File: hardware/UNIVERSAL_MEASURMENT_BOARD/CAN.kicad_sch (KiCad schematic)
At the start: 12 parts, among them U5 ADM3055EBRIZ-RL

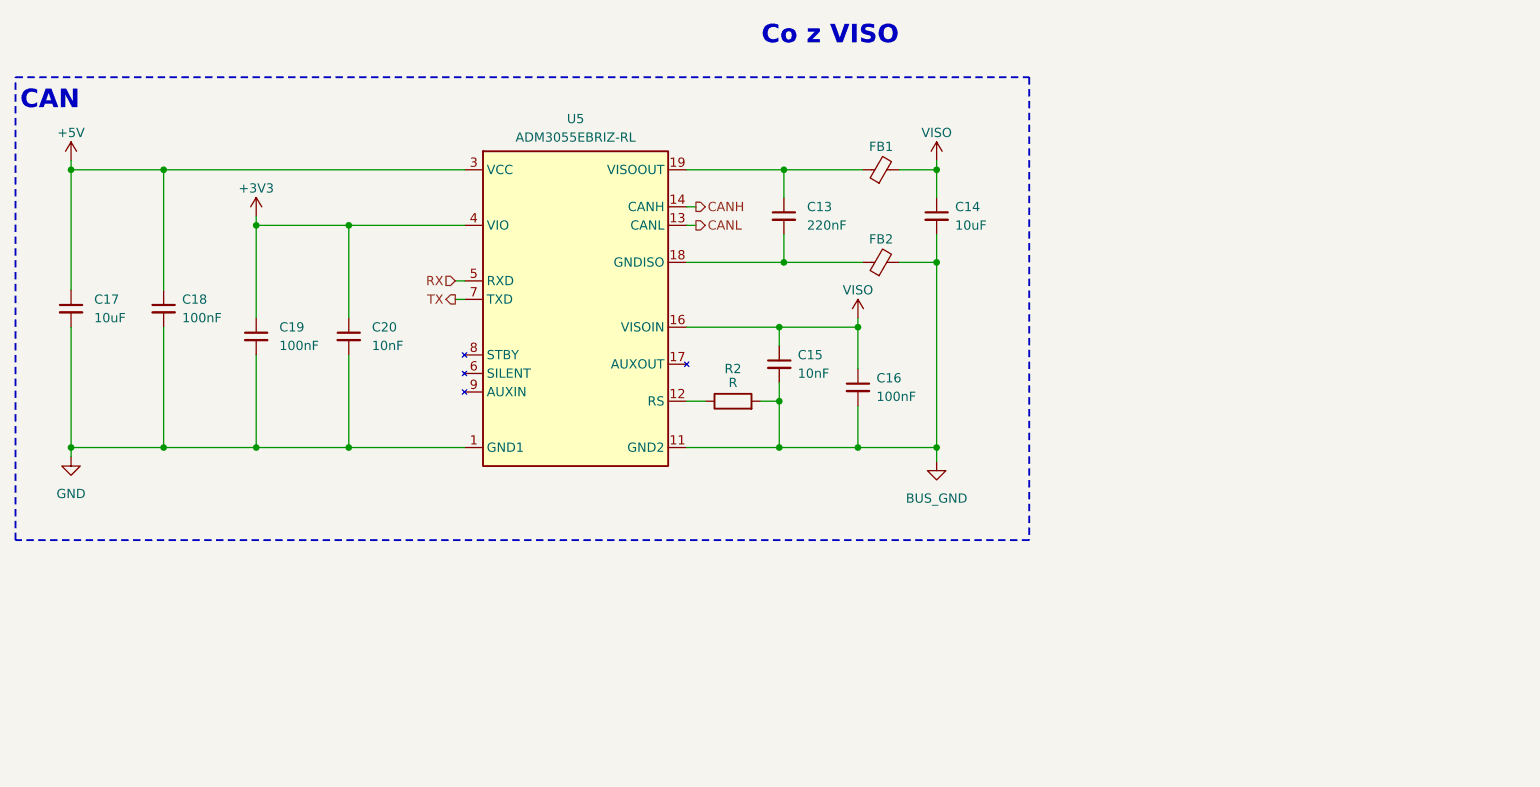
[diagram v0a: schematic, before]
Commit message: continued
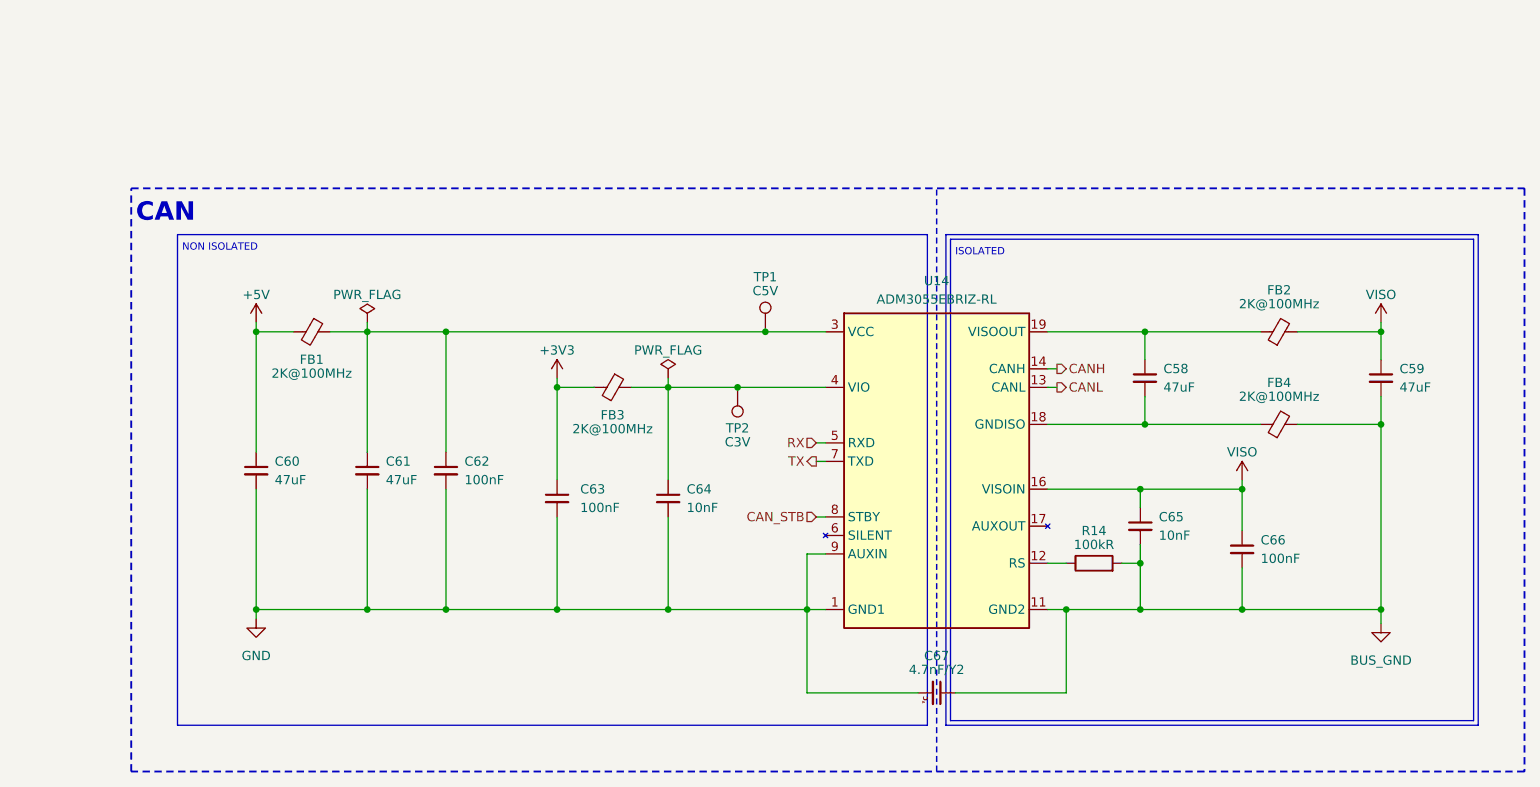
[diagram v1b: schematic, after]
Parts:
- removed FB2: FerriteBead_Small, symbol Device:FerriteBead_Small
- added C61: 47uF, symbol Device:C_Small
- added C67: 4.7nF/Y2, Samacsys:CAPC5728X280N, symbol Samacsys_kicad_sym:S252B222K502CT
- added FB1, FB3, FB4: 2K@100MHz, symbol Device:FerriteBead_Small
- added TP1: C5V, symbol Connector:TestPoint
- added TP2: C3V, symbol Connector:TestPoint
- C58: renamed from C13; value 220nF -> 47uF
- C59: renamed from C14; value 10uF -> 47uF
- C60: renamed from C17; value 10uF -> 47uF
- FB2: renamed from FB1; value FerriteBead_Small -> 2K@100MHz
- R14: renamed from R2; value R -> 100kR
- renumbered C18 to C62, C19 to C63, C20 to C64, C15 to C65, C16 to C66, U5 to U14
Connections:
- net +3V3: now also FB3.2; no longer C64.1, U14.4 (VIO)
- net +5V: now also FB1.2; no longer C62.1, U14.3 (VCC)
- net BUS_GND: now also C67.1, FB4.2
- net GND: now also U14.9 (AUXIN), C61.2, C67.2
- net at C58.2, U14.18 (GNDISO), U14.20 (GNDISO_2): now also FB4.1
- net CAN_STB: now reaches U14.8 (STBY)
- new net: C61.1, C62.1, FB1.1, TP1.1, U14.3 (VCC)
- new net: C64.1, FB3.1, TP2.1, U14.4 (VIO)
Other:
- note added: "ISOLATED"
- note added: "NON ISOLATED"
- note removed: "Co z VISO"
- company: (none) -> PUT Motorsport Formula Student team
- title: (none) -> Universal Measurment Board
- moved on the sheet: C58, C59, C60, C62, C63, C64, C65, C66, FB2, R14
